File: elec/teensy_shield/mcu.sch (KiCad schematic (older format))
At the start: 0 parts

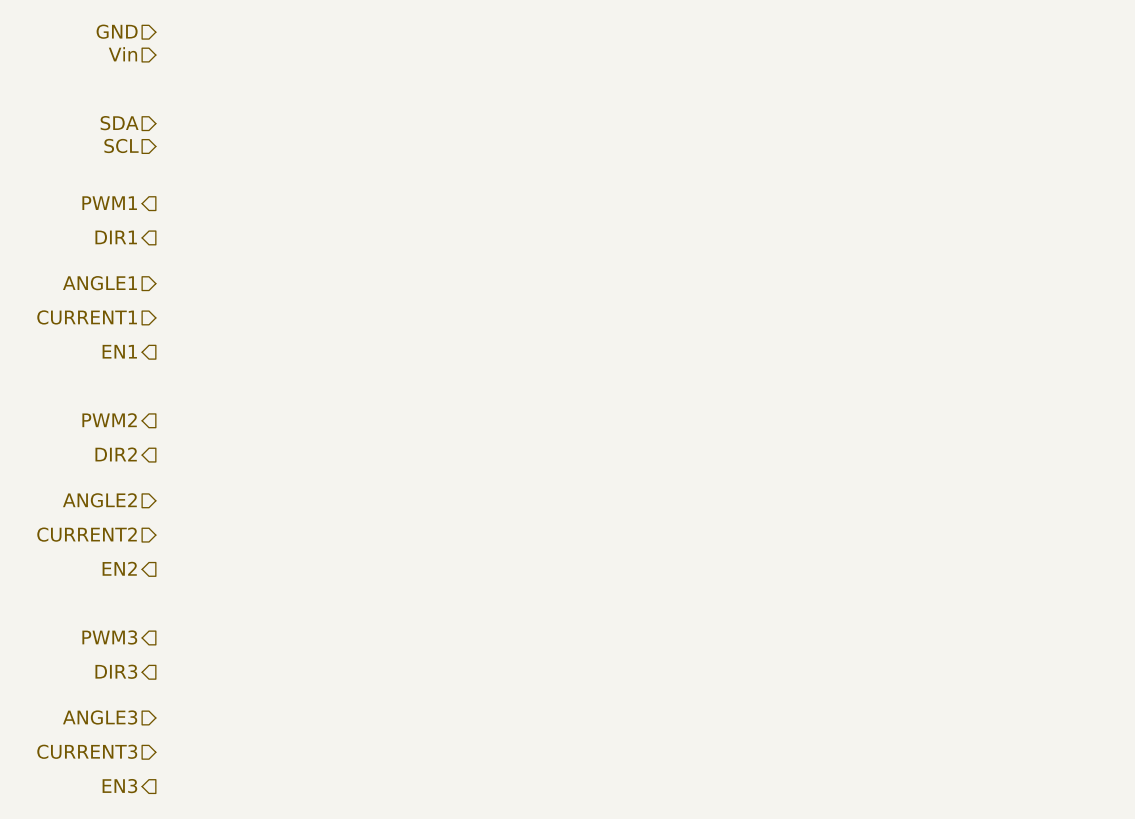
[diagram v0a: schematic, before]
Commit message: Completed new board schematics.
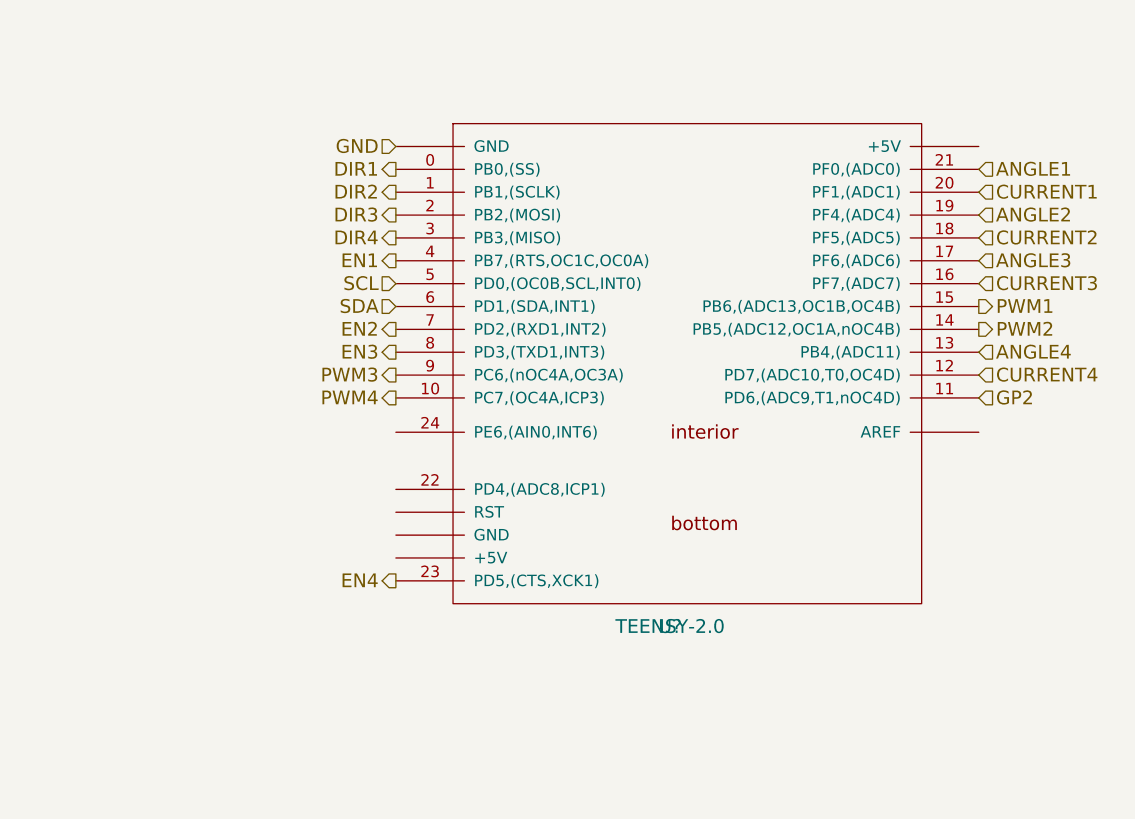
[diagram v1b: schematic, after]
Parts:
- added U?: TEENSY-2.0, symbol TEENSY-2.0
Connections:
- net ANGLE1: now also U?.21 (PF0,(ADC0))
- net ANGLE2: now also U?.19 (PF4,(ADC4))
- net ANGLE3: now also U?.17 (PF6,(ADC6))
- net CURRENT1: now also U?.20 (PF1,(ADC1))
- net CURRENT2: now also U?.18 (PF5,(ADC5))
- net CURRENT3: now also U?.16 (PF7,(ADC7))
- net DIR1: now also U?.0 (PB0,(SS))
- net DIR2: now also U?.1 (PB1,(SCLK))
- net DIR3: now also U?.2 (PB2,(MOSI))
- net EN1: now also U?.4 (PB7,(RTS,OC1C,OC0A))
- net EN2: now also U?.7 (PD2,(RXD1,INT2))
- net EN3: now also U?.8 (PD3,(TXD1,INT3))
- net GND: now also U?.~ (RST)
- net PWM1: now also U?.15 (PB6,(ADC13,OC1B,OC4B))
- net PWM2: now also U?.14 (PB5,(ADC12,OC1A,nOC4B))
- net PWM3: now also U?.9 (PC6,(nOC4A,OC3A))
- net SCL: now also U?.5 (PD0,(OC0B,SCL,INT0))
- net SDA: now also U?.6 (PD1,(SDA,INT1))
- new net ANGLE4: U?.13 (PB4,(ADC11))
- new net CURRENT4: U?.12 (PD7,(ADC10,T0,OC4D))
- new net DIR4: U?.3 (PB3,(MISO))
- new net EN4: U?.23 (PD5,(CTS,XCK1))
- new net GP2: U?.11 (PD6,(ADC9,T1,nOC4D))
- new net PWM4: U?.10 (PC7,(OC4A,ICP3))
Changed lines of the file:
@@
 LIBS:contrib
 LIBS:valves
+LIBS:arduino_shieldsNCL
+LIBS:teensy
+LIBS:pololu
+LIBS:teensy_shield-cache
 EELAYER 24 0
 EELAYER END
 $Descr A4 11693 8268
 encoding utf-8
-Sheet 2 26
+Sheet 2 34
 Title ""
 Date ""
@@
 Comment4 ""
 $EndDescr
-Text HLabel 4100 1800 0    60   Input ~ 0
+Text HLabel 5150 2300 0    60   Input ~ 0
 GND
-Text HLabel 4100 1900 0    60   Input ~ 0
-Vin
-Text HLabel 4100 2550 0    60   Output ~ 0
+Text HLabel 7700 3000 2    60   Output ~ 0
 PWM1
-Text HLabel 4100 2700 0    60   Output ~ 0
+Text HLabel 5150 2400 0    60   Output ~ 0
 DIR1
-Text HLabel 4100 2900 0    60   Input ~ 0
+Text HLabel 7700 2400 2    60   Input ~ 0
 ANGLE1
-Text HLabel 4100 3050 0    60   Input ~ 0
+Text HLabel 7700 2500 2    60   Input ~ 0
 CURRENT1
-Text HLabel 4100 3200 0    60   Output ~ 0
+Text HLabel 5150 2800 0    60   Output ~ 0
 EN1
-Text HLabel 4100 3500 0    60   Output ~ 0
+Text HLabel 7700 3100 2    60   Output ~ 0
 PWM2
-Text HLabel 4100 3650 0    60   Output ~ 0
+Text HLabel 5150 2500 0    60   Output ~ 0
 DIR2
-Text HLabel 4100 3850 0    60   Input ~ 0
+Text HLabel 7700 2600 2    60   Input ~ 0
 ANGLE2
-Text HLabel 4100 4000 0    60   Input ~ 0
+Text HLabel 7700 2700 2    60   Input ~ 0
 CURRENT2
-Text HLabel 4100 4150 0    60   Output ~ 0
+Text HLabel 5150 3100 0    60   Output ~ 0
 EN2
-Text HLabel 4100 4450 0    60   Output ~ 0
+Text HLabel 5150 3300 0    60   Output ~ 0
 PWM3
-Text HLabel 4100 4600 0    60   Output ~ 0
+Text HLabel 5150 2600 0    60   Output ~ 0
 DIR3
-Text HLabel 4100 4800 0    60   Input ~ 0
+Text HLabel 7700 2800 2    60   Input ~ 0
 ANGLE3
-Text HLabel 4100 4950 0    60   Input ~ 0
+Text HLabel 7700 2900 2    60   Input ~ 0
 CURRENT3
-Text HLabel 4100 5100 0    60   Output ~ 0
+Text HLabel 5150 3200 0    60   Output ~ 0
 EN3
-Text HLabel 4100 2200 0    60   Input ~ 0
+Text HLabel 5150 3000 0    60   Input ~ 0
 SDA
-Text HLabel 4100 2300 0    60   Input ~ 0
+Text HLabel 5150 2900 0    60   Input ~ 0
 SCL
+$Comp
+L TEENSY-2.0 U?
+U 1 1 55E7159A
+P 6350 3250
+F 0 "U?" H 6350 2100 60  0000 C CNN
+F 1 "TEENSY-2.0" H 6350 2100 60  0000 C CNN
+F 2 "" H 6350 2100 60  0000 C CNN
+F 3 "" H 6350 2100 60  0000 C CNN
+	1    6350 3250
+	1    0    0    -1
+$EndComp
+Text HLabel 5150 3400 0    60   Output ~ 0
+PWM4
+Text HLabel 5150 2700 0    60   Output ~ 0
+DIR4
+Text HLabel 7700 3200 2    60   Input ~ 0
+ANGLE4
+Text HLabel 7700 3300 2    60   Input ~ 0
+CURRENT4
+Text HLabel 5150 4200 0    60   Output ~ 0
+EN4
+Text HLabel 7700 3400 2    60   Input ~ 0
+GP2
 $EndSCHEMATC

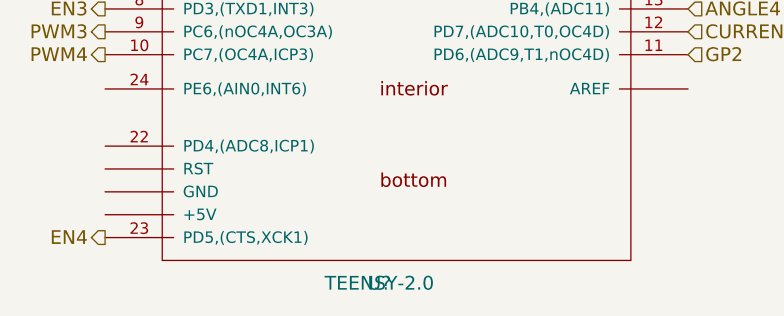
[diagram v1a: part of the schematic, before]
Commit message: Elec ?
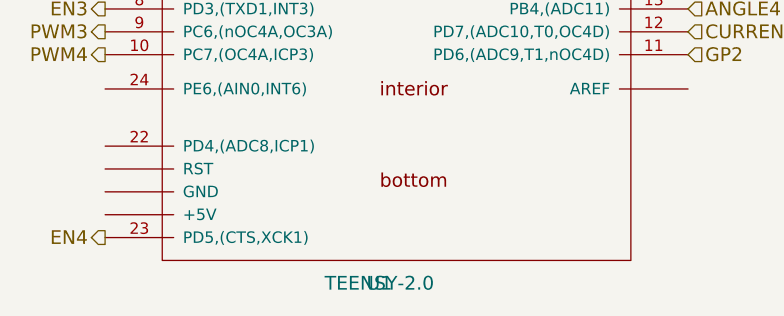
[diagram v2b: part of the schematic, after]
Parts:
- gave numbers to parts that had none: 1
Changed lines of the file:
@@
 SCL
 $Comp
-L TEENSY-2.0 U?
+L TEENSY-2.0 U1
 U 1 1 55E7159A
 P 6350 3250
-F 0 "U?" H 6350 2100 60  0000 C CNN
+F 0 "U1" H 6350 2100 60  0000 C CNN
 F 1 "TEENSY-2.0" H 6350 2100 60  0000 C CNN
 F 2 "" H 6350 2100 60  0000 C CNN
